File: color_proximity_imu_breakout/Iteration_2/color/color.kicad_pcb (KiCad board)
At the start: 2 copper layers, 13 x 20 mm, 19 parts, among them IC2 ISL29125IROZ-T7, J1 Conn_01x10, J2 Conn_01x10

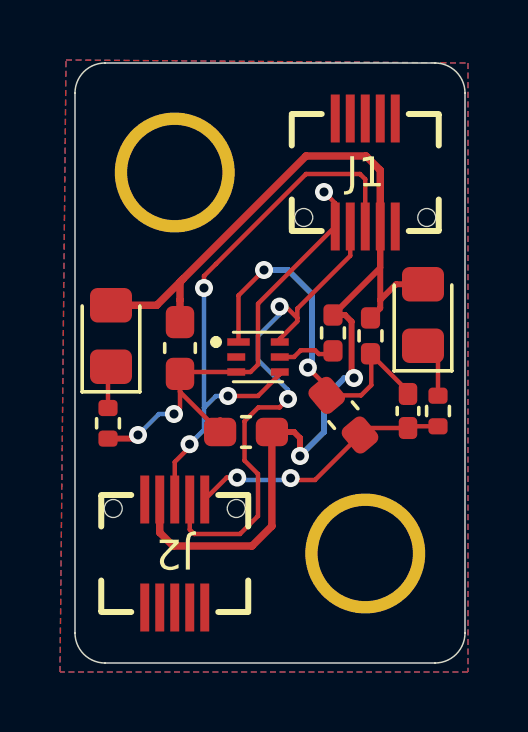
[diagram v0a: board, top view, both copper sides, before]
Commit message: updated production files
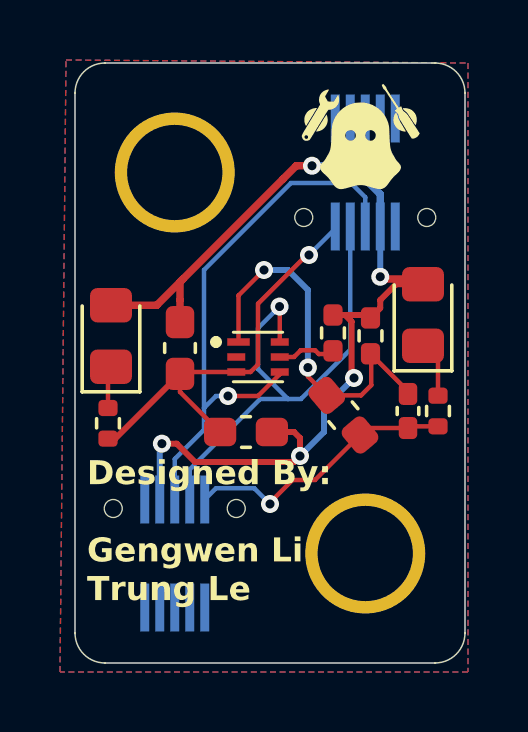
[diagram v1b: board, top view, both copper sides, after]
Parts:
- removed the G*** at (105.2, 121.6)
- removed the G*** at (111.4, 113.0)
- G***: moved to F.Cu
- J1, J2: moved to B.Cu
- moved G*** 8.91 mm to (111.4, 106.6), turned to 0 degrees
- moved G*** 3.46 mm to (108.3, 113.9), turned to -145 degrees
- turned C1 to 180 degrees
- turned C2 to -90 degrees
- turned J1 to 180 degrees
- turned J2 to 0 degrees
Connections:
- C1 pad 1: GND -> +3.3V
- C1 pad 2: +3.3V -> GND
- C2 pad 1: GND -> +3.3V
- C2 pad 2: +3.3V -> GND
- J1 pad 10: unconnected-(J1-Pin_10-Pad10) -> GND
- J1 pad 6: GND -> unconnected-(J1-Pin_6-Pad6)
- J1 pad 7: /scl -> +3.3V
- J1 pad 9: +3.3V -> /scl
- J2 pad 10: unconnected-(J2-Pin_10-Pad10) -> GND
- J2 pad 6: GND -> unconnected-(J2-Pin_6-Pad6)
- J2 pad 7: /scl -> +3.3V
- J2 pad 9: +3.3V -> /scl
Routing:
- net +3.3V: track 40.1 -> 36.0 mm, vias 2 -> 5
- net GND: track 25.1 -> 23.4 mm, vias 5 -> 2
- net /scl: track 18.1 -> 17.1 mm, vias 2 -> 1
- net /sda: track 19.6 -> 19.1 mm, vias 3 -> 1
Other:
- board text added: "Designed By: Gengwen Li Trung Le"
- board text removed: "Designed By Gengwen Li Trung Le"
